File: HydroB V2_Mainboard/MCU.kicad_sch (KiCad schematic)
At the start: 17 parts, among them SW1 SW_Push, SW2 SW_Push, U1 ESP32-S3-WROOM-1-N16R2

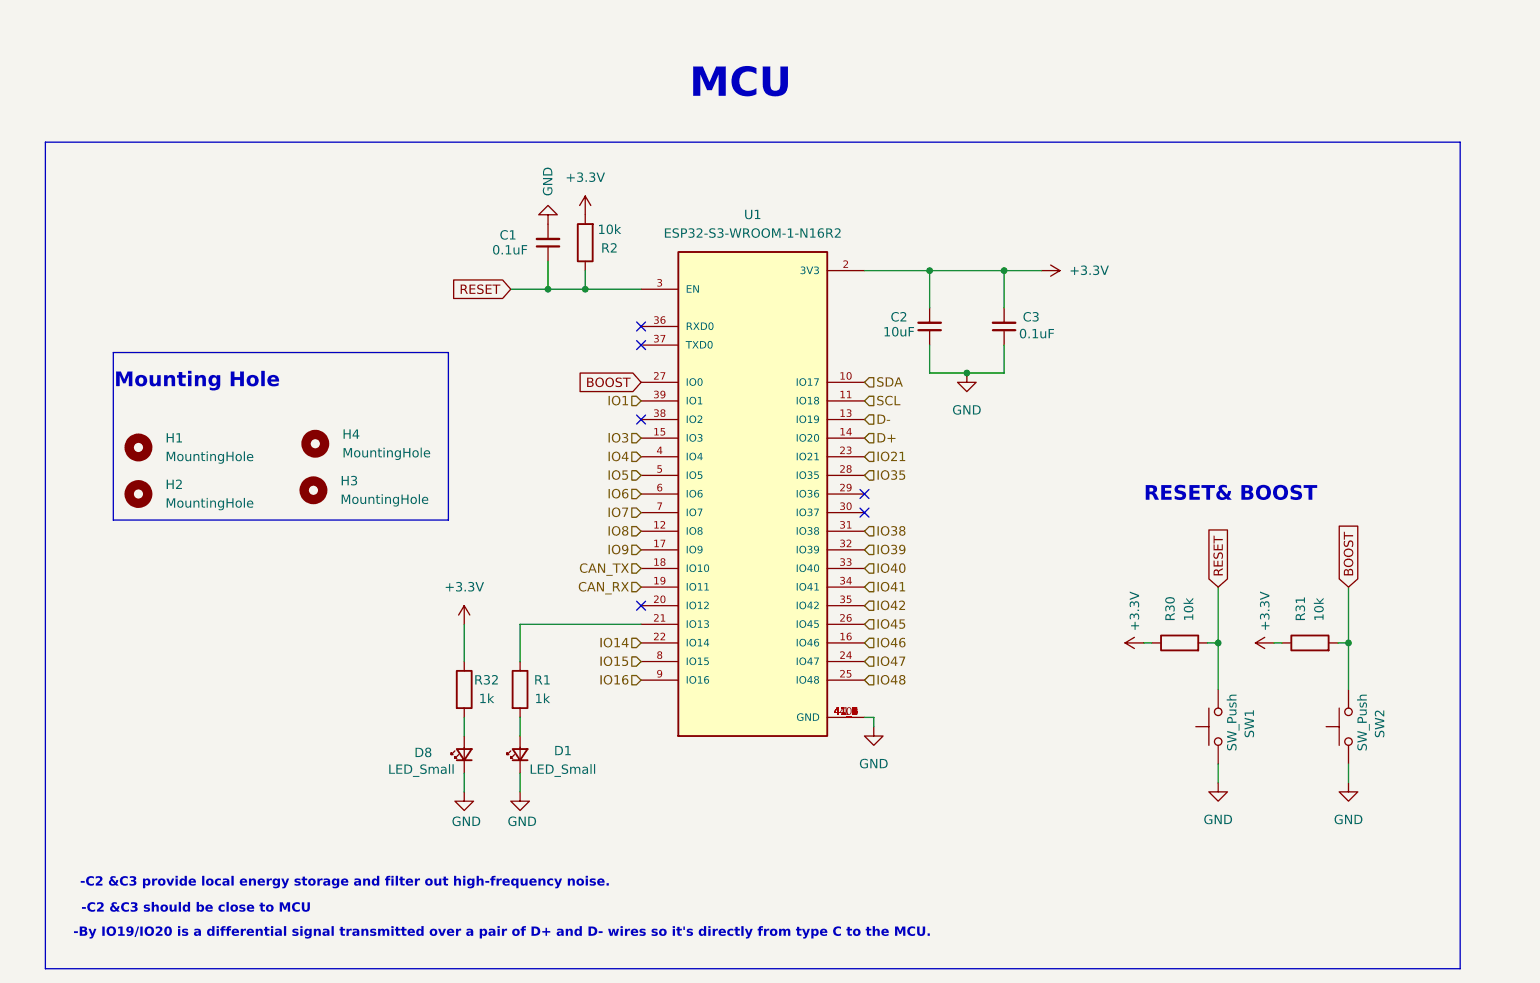
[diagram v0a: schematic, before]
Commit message: Schematic mainboard update
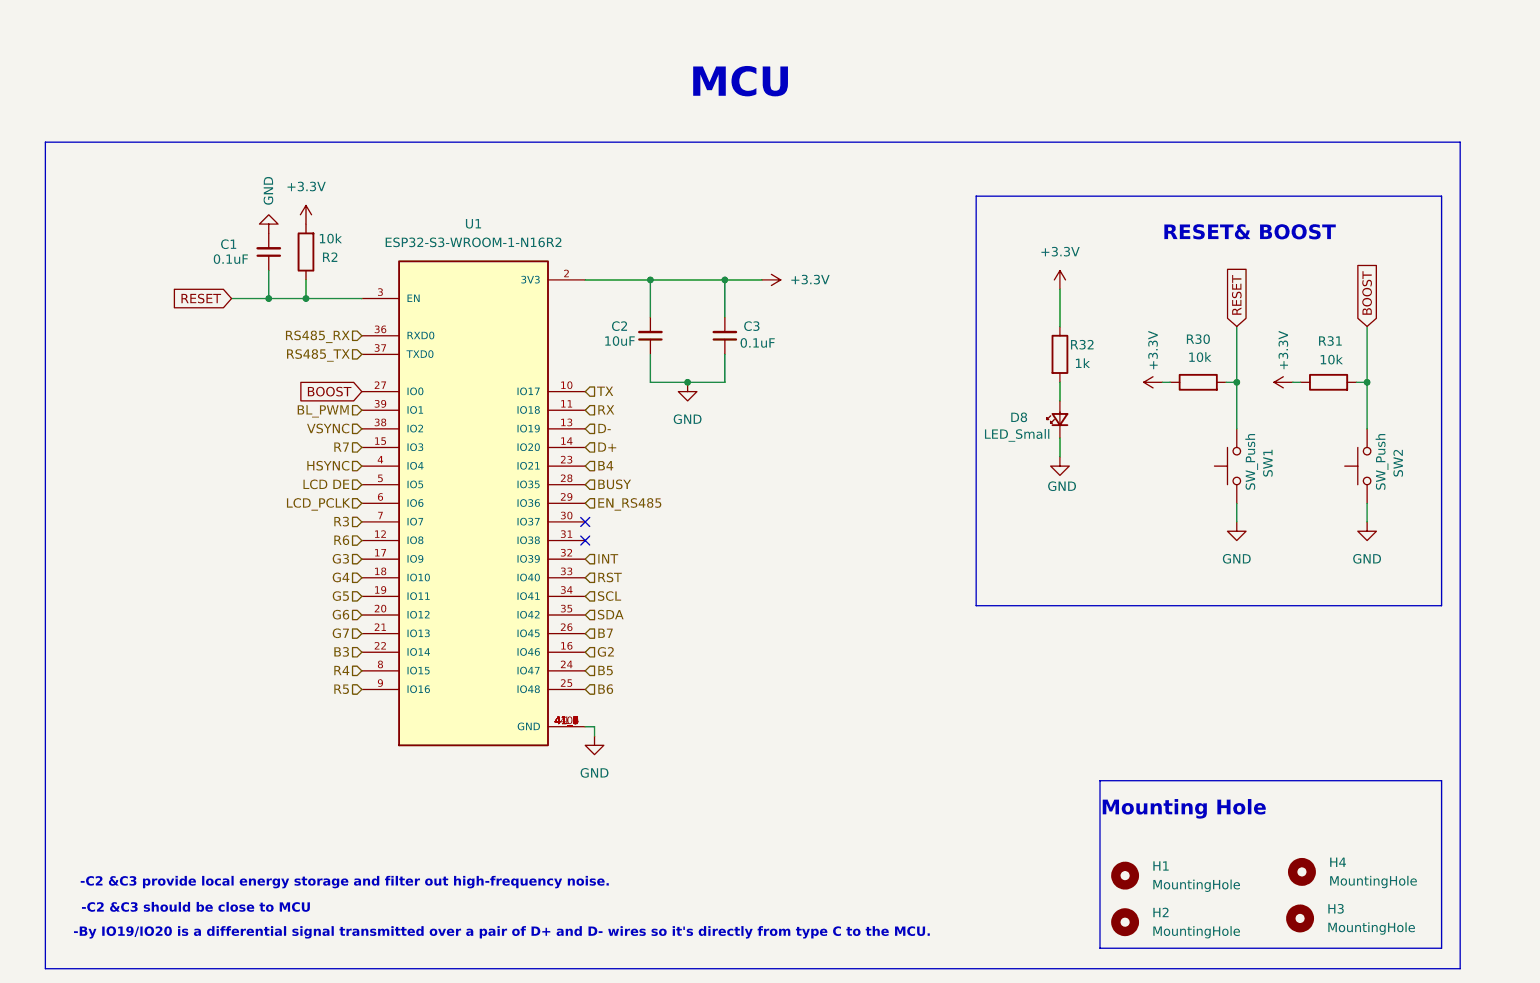
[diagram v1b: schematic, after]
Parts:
- removed D1: LED_Small, LED_SMD:LED_0805_2012Metric, symbol Device:LED_Small
- removed R1: 1k, Resistor_SMD:R_0603_1608Metric, symbol Device:R
- SW1, SW2: footprint Button_Switch_SMD:SW_Push_1P1T_NO_CK_KMR2 -> Button_Switch_SMD:SW_Push_SPST_NO_Alps_SKRK
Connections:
- net IO41 is gone; now on net SCL: U1.34 (IO41)
- net IO42 is gone; now on net SDA: U1.35 (IO42)
- net SCL: no longer U1.11 (IO18)
- net SDA: no longer U1.10 (IO17)
- net G6: now reaches U1.20 (IO12)
- net G7: now reaches U1.21 (IO13)
- net EN_RS485: now reaches U1.29 (IO36)
- net RS485_RX: now reaches U1.36 (RXD0)
- net RS485_TX: now reaches U1.37 (TXD0)
- net VSYNC: now reaches U1.38 (IO2)
- net CAN_RX renamed G5
- net CAN_TX renamed G4
- net IO1 renamed BL_PWM
- net IO14 renamed B3
- net IO15 renamed R4
- net IO16 renamed R5
- net IO21 renamed B4
- net IO3 renamed R7
- net IO35 renamed BUSY
- net IO38: no longer names the net of U1.31 (IO38)
- net IO39 renamed INT
- net IO4 renamed HSYNC
- net IO40 renamed RST
- net IO45 renamed B7
- net IO46 renamed G2
- net IO47 renamed B5
- net IO48 renamed B6
- net IO5 renamed LCD DE
- net IO6 renamed LCD_PCLK
- net IO7 renamed R3
- net IO8 renamed R6
- net IO9 renamed G3
- new net RX: U1.11 (IO18)
- new net TX: U1.10 (IO17)
- no-connect marks 6 -> 2
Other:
- moved on the sheet: C1, C2, C3, D8, H1, H2, H3, H4, R2, R30, R31, R32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

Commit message: Mainboard schematic update
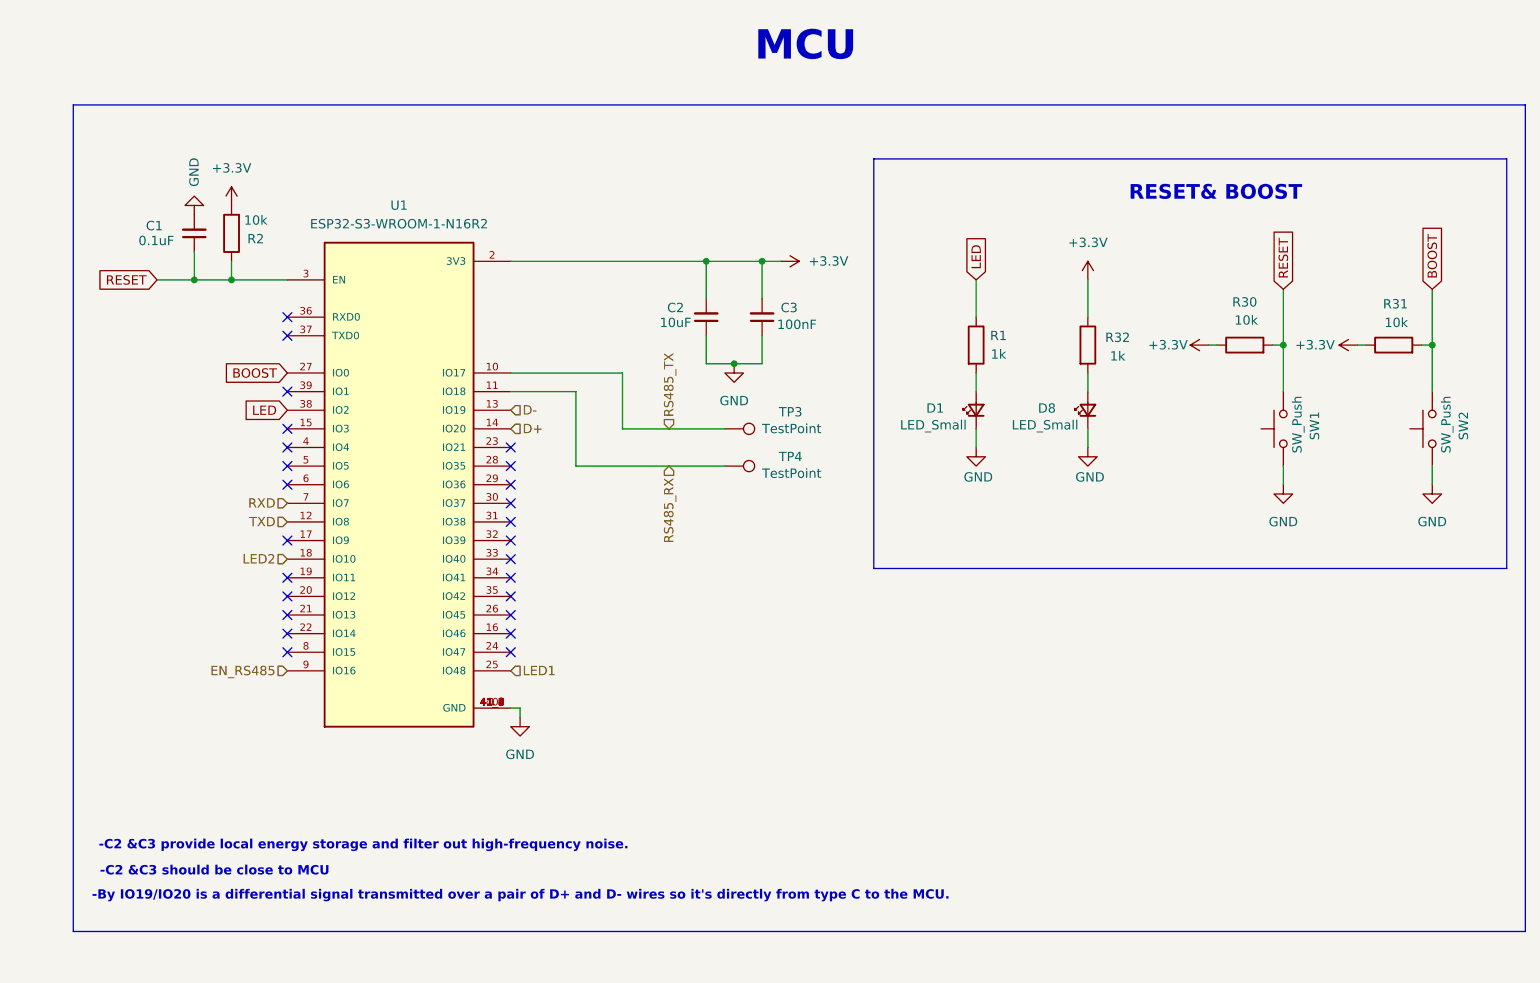
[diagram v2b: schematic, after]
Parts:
- removed H1, H2, H3, H4: MountingHole, MountingHole:MountingHole_3mm_Pad_Via, symbol Mechanical:MountingHole
- added D1: LED_Small, LED_SMD:LED_0805_2012Metric, symbol Device:LED_Small
- added R1: 1k, Resistor_SMD:R_0603_1608Metric, symbol Device:R
- added TP3, TP4: TestPoint, TestPoint:TestPoint_Loop_D1.80mm_Drill1.0mm_Beaded, symbol Connector:TestPoint
- C3: value 0.1uF -> 100nF
- SW1: footprint Button_Switch_SMD:SW_Push_SPST_NO_Alps_SKRK -> Button_Switch_THT:SW_Tactile_SPST_Angled_PTS645Vx39-2LFS
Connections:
- net R5 is gone; now on net EN_RS485: U1.9 (IO16)
- net RX is gone; now on net RS485_RX: U1.11 (IO18)
- net TX is gone; now on net RS485_TX: U1.10 (IO17)
- net EN_RS485: no longer U1.29 (IO36)
- net GND: now also D1.1 (K)
- net RS485_RX: now also TP4.1; no longer U1.36 (RXD0)
- net RS485_TX: now also TP3.1; no longer U1.37 (TXD0)
- net B3: no longer names the net of U1.22 (IO14)
- net B4: no longer names the net of U1.23 (IO21)
- net B5: no longer names the net of U1.24 (IO47)
- net B6 renamed LED1
- net B7: no longer names the net of U1.26 (IO45)
- net BL_PWM: no longer names the net of U1.39 (IO1)
- net BUSY: no longer names the net of U1.28 (IO35)
- net G2: no longer names the net of U1.16 (IO46)
- net G3: no longer names the net of U1.17 (IO9)
- net G4 renamed LED2
- net G5: no longer names the net of U1.19 (IO11)
- net G6: no longer names the net of U1.20 (IO12)
- net G7: no longer names the net of U1.21 (IO13)
- net HSYNC: no longer names the net of U1.4 (IO4)
- net INT: no longer names the net of U1.32 (IO39)
- net LCD DE: no longer names the net of U1.5 (IO5)
- net LCD_PCLK: no longer names the net of U1.6 (IO6)
- net R3 renamed RXD
- net R4: no longer names the net of U1.8 (IO15)
- net R6 renamed TXD
- net R7: no longer names the net of U1.15 (IO3)
- net RST: no longer names the net of U1.33 (IO40)
- net SCL: no longer names the net of U1.34 (IO41)
- net SDA: no longer names the net of U1.35 (IO42)
- net VSYNC renamed LED
- net LED: now also R1.1
- new net: D1.2 (A), R1.2
- no-connect marks 2 -> 25
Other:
- note removed: "Mounting Hole"
- moved on the sheet: C1, C2, C3, D8, R2, R30, R31, R32, SW1, SW2, U1
